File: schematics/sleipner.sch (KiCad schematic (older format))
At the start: 129 parts, among them J1 Conn_01x04_Male, J10 AudioJack3, J11 AudioJack3, J12 AudioJack3, J13 AudioJack3, J2 Barrel_Jack_Switch, J3 AudioJack3, J4 AudioJack3, J5 AudioJack3, J6 AudioJack3, J7 AudioJack3, J8 AudioJack3, J9 AudioJack3, Q1 BC337, Q2 BC337, Q3 BC337, Q4 BC337, Q5 BC337, Q6 BC337, Q7 BC337, Q8 BC337, Q9 BC337, SW1 SW_DIP_x02, SW10 SW_DIP_x02, SW11 Rotary_Encoder, SW12 SW_DIP_x02, SW13 SW_DIP_x02, SW14 SW_DIP_x02, SW15 SW_DIP_x02, SW16 SW_DIP_x02, SW17 SW_DIP_x02, SW18 SW_DIP_x02, SW19 SW_DIP_x02, SW2 SW_DIP_x02, SW3 SW_DIP_x02, SW4 SW_DIP_x02, SW5 SW_DIP_x02, SW6 SW_DIP_x02, SW7 SW_DIP_x02, SW8 SW_DIP_x02, SW9 SW_DIP_x02, U1 L7805, U2 ATmega32-16PU, U3 L7812, U4 74LS259, U5 MCP4922-EP, U6 TLC274, Y1 16 MHz

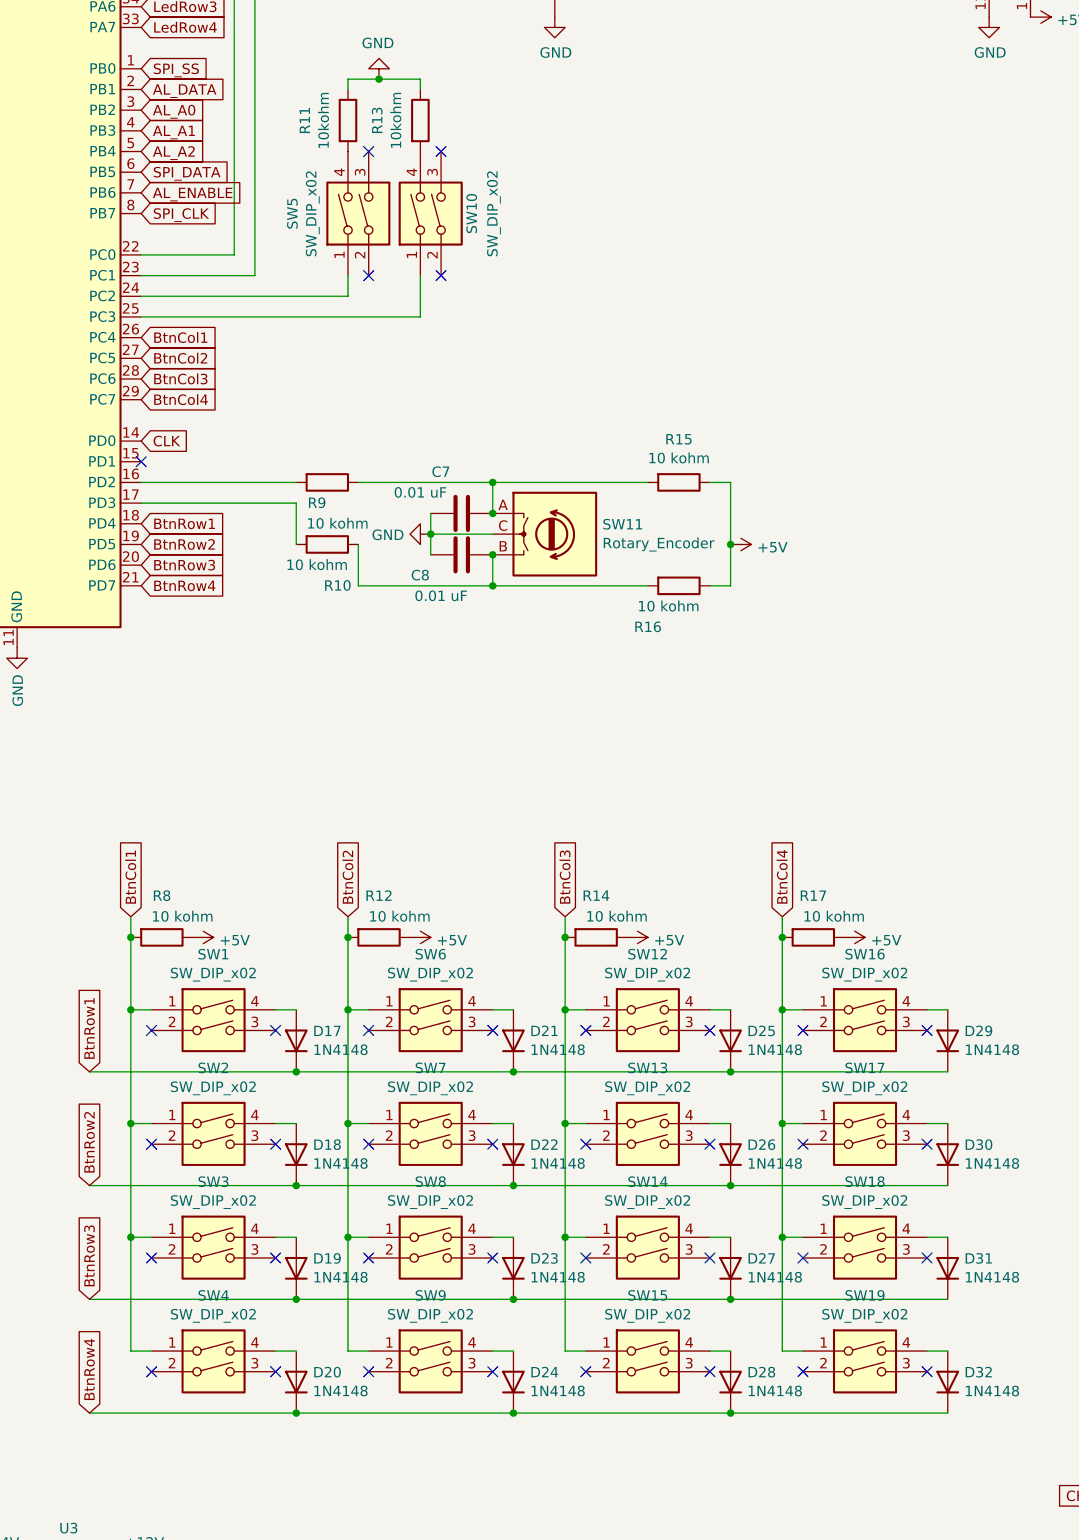
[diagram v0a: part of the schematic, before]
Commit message: Update schematics and add PCB layout
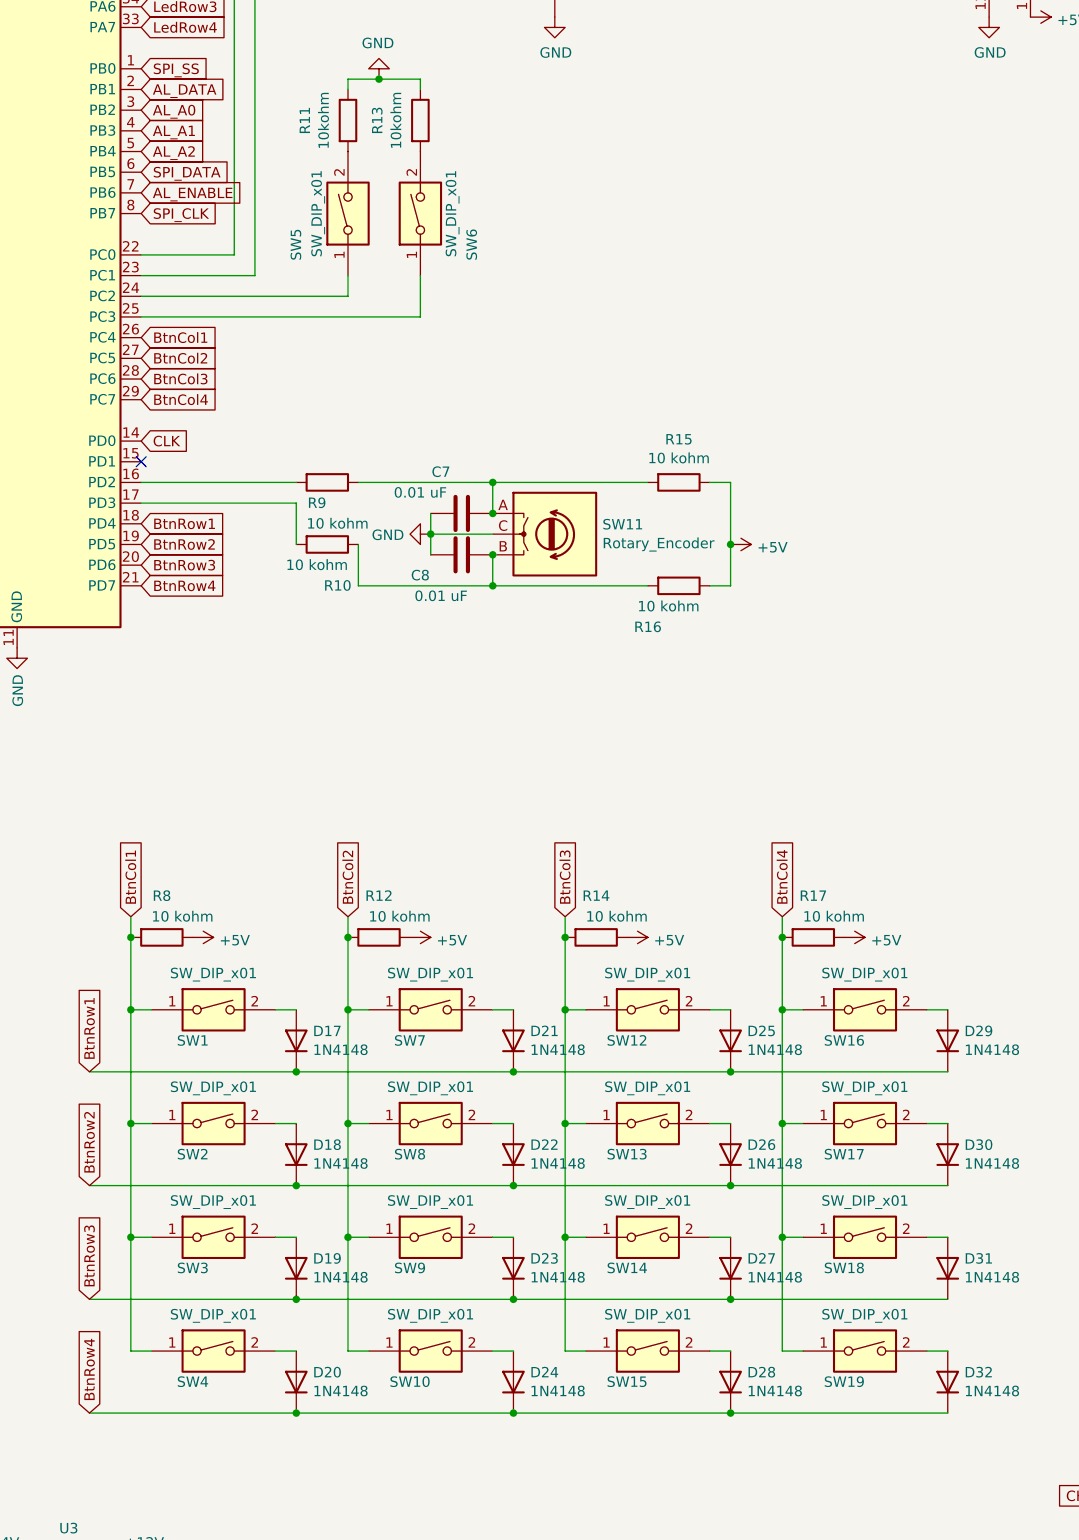
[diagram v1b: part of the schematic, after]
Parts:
- removed SW1, SW10, SW12, SW13, SW14, SW15, SW16, SW17, SW18, SW19, SW2, SW3, SW4, SW5, SW6, SW7, SW8, SW9: SW_DIP_x02, Button_Switch_THT:SW_PUSH-12mm, symbol Switch:SW_DIP_x02
- added SW1, SW10, SW12, SW13, SW14, SW15, SW16, SW17, SW18, SW19, SW2, SW3, SW4, SW5, SW6, SW7, SW8, SW9: SW_DIP_x01, Button_Switch_THT:SW_PUSH-12mm, symbol Switch:SW_DIP_x01
- J10, J11, J12, J13, J3, J4, J5, J6, J7, J8, J9: footprint (none) -> 3.5mmJack:3.55mmJack
- U4: footprint (none) -> Package_DIP:DIP-16_W7.62mm
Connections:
- net BtnCol1: now also SW1.1, SW2.1, SW3.1, SW4.1
- net BtnCol2: now also SW10.1, SW7.1, SW8.1, SW9.1
- net BtnCol3: now also SW12.1, SW13.1, SW14.1, SW15.1
- net BtnCol4: now also SW16.1, SW17.1, SW18.1, SW19.1
- net at U2.24 (PC2): now also SW5.1
- net at U2.25 (PC3): now also SW6.1
- net at D21.2 (A): now also SW7.2
- net at D17.2 (A): now also SW1.2
- net at D25.2 (A): now also SW12.2
- net at D29.2 (A): now also SW16.2
- net at D19.2 (A): now also SW3.2
- net at D23.2 (A): now also SW9.2
- net at D27.2 (A): now also SW14.2
- net at D31.2 (A): now also SW18.2
- net at D18.2 (A): now also SW2.2
- net at D22.2 (A): now also SW8.2
- net at D26.2 (A): now also SW13.2
- net at D30.2 (A): now also SW17.2
- net at D20.2 (A): now also SW4.2
- net at D24.2 (A): now also SW10.2
- net at D28.2 (A): now also SW15.2
- net at D32.2 (A): now also SW19.2
- net at R11.2: now also SW5.2
- net at R13.2: now also SW6.2
- no-connect marks 51 -> 15

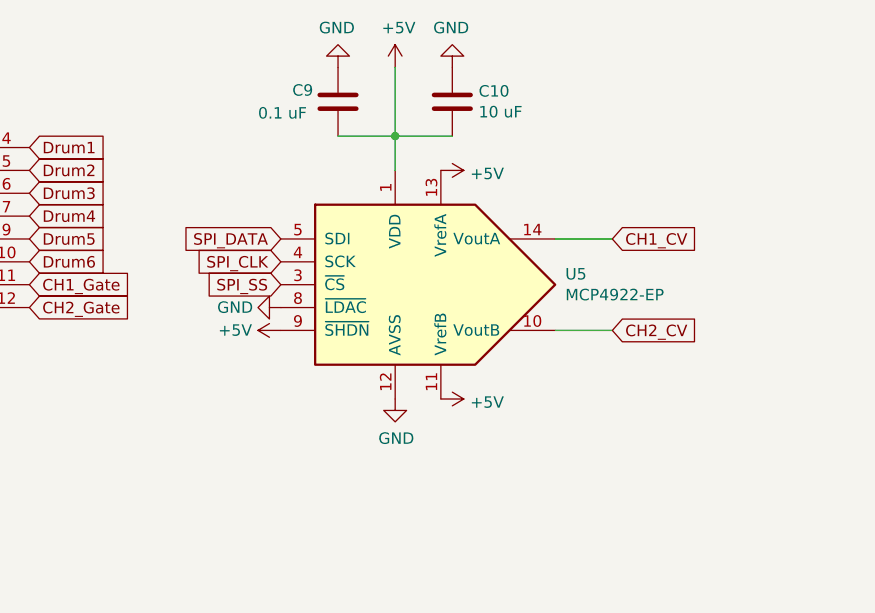
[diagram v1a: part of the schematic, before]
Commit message: Redo the PCB
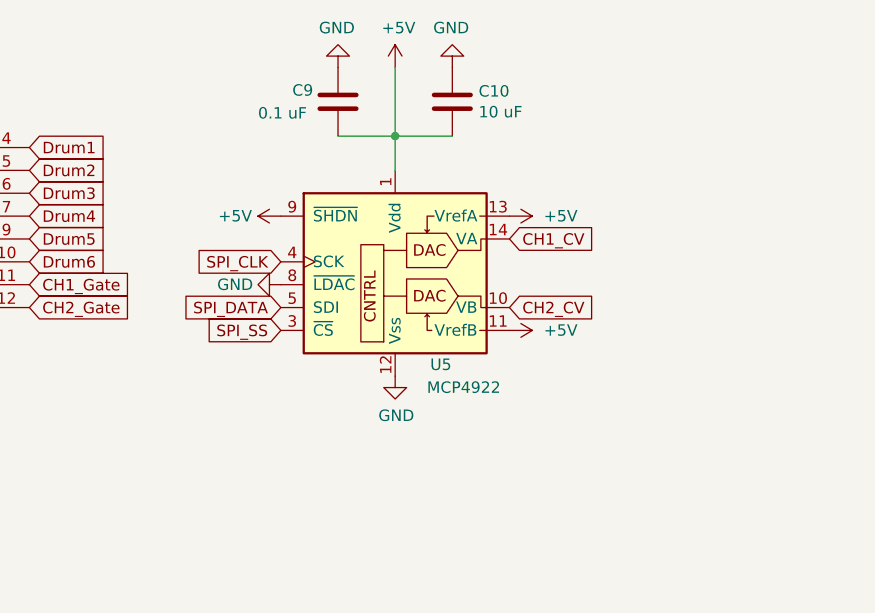
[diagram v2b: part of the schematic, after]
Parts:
- removed U5: MCP4922-EP, mcp4922:DIP254P762X533-14, symbol Analog_DAC:MCP4922-EP
- added U5: MCP4922, Package_DIP:DIP-14_W7.62mm, symbol Analog_DAC:MCP4922
- U6: footprint tlc274:DIP794W45P254L1969H508Q14 -> Package_DIP:DIP-14_W7.62mm
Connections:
- net +5V: now also U5.1 (Vdd), U5.11 (VrefB), U5.13 (VrefA), U5.9 (~SHDN)
- net CH1_CV: now also U5.14 (VA)
- net CH2_CV: now also U5.10 (VB)
- net GND: now also U5.12 (Vss), U5.8 (~LDAC)
- net SPI_CLK: now also U5.4 (SCK)
- net SPI_DATA: now also U5.5 (SDI)
- net SPI_SS: now also U5.3 (~CS)
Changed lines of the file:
@@
-$EndComp
-$Comp
-L Analog_DAC:MCP4922-EP U5
-U 1 1 60919F79
-P 7800 2350
-F 0 "U5" H 8444 2396 50  0000 L CNN
-F 1 "MCP4922-EP" H 8444 2305 50  0000 L CNN
-F 2 "mcp4922:DIP254P762X533-14" H 7800 2350 50  0001 C CIN
-F 3 "http://ww1.microchip.com/downloads/en/devicedoc/21897a.pdf" H 7800 2350 50  0001 C CNN
-	1    7800 2350
-	1    0    0    -1
 $EndComp
 $Comp
@@
 F 0 "U6" H 8750 10400 50  0000 C CNN
 F 1 "TLC274" H 8800 10300 50  0000 C CNN
-F 2 "tlc274:DIP794W45P254L1969H508Q14" H 8650 10200 50  0001 C CNN
+F 2 "Package_DIP:DIP-14_W7.62mm" H 8650 10200 50  0001 C CNN
 F 3 "http://www.ti.com/lit/ds/symlink/tlc274.pdf" H 8750 10300 50  0001 C CNN
 	1    8700 10100
@@
 F 0 "U6" H 8658 10146 50  0000 L CNN
 F 1 "TLC274" H 8658 10055 50  0000 L CNN
-F 2 "tlc274:DIP794W45P254L1969H508Q14" H 8650 10200 50  0001 C CNN
+F 2 "Package_DIP:DIP-14_W7.62mm" H 8650 10200 50  0001 C CNN
 F 3 "http://www.ti.com/lit/ds/symlink/tlc274.pdf" H 8750 10300 50  0001 C CNN
 	5    8700 10100
@@
 F 0 "U6" H 10500 10400 50  0000 C CNN
 F 1 "TLC274" H 10550 10300 50  0000 C CNN
-F 2 "tlc274:DIP794W45P254L1969H508Q14" H 10400 10200 50  0001 C CNN
+F 2 "Package_DIP:DIP-14_W7.62mm" H 10400 10200 50  0001 C CNN
 F 3 "http://www.ti.com/lit/ds/symlink/tlc274.pdf" H 10500 10300 50  0001 C CNN
 	2    10450 10100
@@
 L power:GND #PWR030
 U 1 1 6149602B
-P 7700 2850
-F 0 "#PWR030" H 7700 2600 50  0001 C CNN
-F 1 "GND" H 7705 2677 50  0000 C CNN
-F 2 "" H 7700 2850 50  0001 C CNN
-F 3 "" H 7700 2850 50  0001 C CNN
-	1    7700 2850
+P 7700 2750
+F 0 "#PWR030" H 7700 2500 50  0001 C CNN
+F 1 "GND" H 7705 2577 50  0000 C CNN
+F 2 "" H 7700 2750 50  0001 C CNN
+F 3 "" H 7700 2750 50  0001 C CNN
+	1    7700 2750
 	1    0    0    -1
 $EndComp
@@
 $EndComp
 $Comp
-L power:GND #PWR033
+L power:GND #PWR031
 U 1 1 6157DF10
 P 7950 1400
-F 0 "#PWR033" H 7950 1150 50  0001 C CNN
+F 0 "#PWR031" H 7950 1150 50  0001 C CNN
 F 1 "GND" H 7955 1227 50  0000 C CNN
 F 2 "" H 7950 1400 50  0001 C CNN
@@
 	1    0    0    -1
 $EndComp
-Text GLabel 8650 2150 2    50   Input ~ 0
+Text GLabel 8200 2150 2    50   Input ~ 0
 CH1_CV
-Text GLabel 8650 2550 2    50   Input ~ 0
+Text GLabel 8200 2450 2    50   Input ~ 0
 CH2_CV
 Text GLabel 14400 4600 1    50   Input ~ 0
@@
 Text GLabel 8400 10000 0    50   Input ~ 0
 CH1_CV
-Wire Wire Line
-	8400 2550 8650 2550
-Wire Wire Line
-	8400 2150 8650 2150
-$Comp
-L power:+5V #PWR031
+$Comp
+L power:+5V #PWR032
 U 1 1 63C2EF82
-P 7900 1850
-F 0 "#PWR031" H 7900 1700 50  0001 C CNN
-F 1 "+5V" V 7915 1978 50  0000 L CNN
-F 2 "" H 7900 1850 50  0001 C CNN
-F 3 "" H 7900 1850 50  0001 C CNN
-	1    7900 1850
-	0    1    1    0
-$EndComp
-$Comp
-L power:+5V #PWR032
+P 8200 2050
+F 0 "#PWR032" H 8200 1900 50  0001 C CNN
+F 1 "+5V" V 8200 2200 50  0000 L CNN
+F 2 "" H 8200 2050 50  0001 C CNN
+F 3 "" H 8200 2050 50  0001 C CNN
+	1    8200 2050
+	0    1    1    0
+$EndComp
+$Comp
+L power:+5V #PWR033
 U 1 1 63C4DC09
-P 7900 2850
-F 0 "#PWR032" H 7900 2700 50  0001 C CNN
-F 1 "+5V" V 7915 2978 50  0000 L CNN
-F 2 "" H 7900 2850 50  0001 C CNN
-F 3 "" H 7900 2850 50  0001 C CNN
-	1    7900 2850
+P 8200 2550
+F 0 "#PWR033" H 8200 2400 50  0001 C CNN
+F 1 "+5V" V 8200 2700 50  0000 L CNN
+F 2 "" H 8200 2550 50  0001 C CNN
+F 3 "" H 8200 2550 50  0001 C CNN
+	1    8200 2550
 	0    1    1    0
 $EndComp
@@
 	7700 1400 7700 1700
 $Comp
-L power:GND #PWR026
+L power:GND #PWR027
 U 1 1 60B62D9D
-P 7200 2450
-F 0 "#PWR026" H 7200 2200 50  0001 C CNN
-F 1 "GND" V 7200 2250 50  0000 C CNN
-F 2 "" H 7200 2450 50  0001 C CNN
-F 3 "" H 7200 2450 50  0001 C CNN
-	1    7200 2450
-	0    1    1    0
-$EndComp
-$Comp
-L power:+5V #PWR027
+P 7200 2350
+F 0 "#PWR027" H 7200 2100 50  0001 C CNN
+F 1 "GND" V 7200 2150 50  0000 C CNN
+F 2 "" H 7200 2350 50  0001 C CNN
+F 3 "" H 7200 2350 50  0001 C CNN
+	1    7200 2350
+	0    1    1    0
+$EndComp
+$Comp
+L power:+5V #PWR026
 U 1 1 60B64956
-P 7200 2550
-F 0 "#PWR027" H 7200 2400 50  0001 C CNN
-F 1 "+5V" V 7200 2750 50  0000 C CNN
-F 2 "" H 7200 2550 50  0001 C CNN
-F 3 "" H 7200 2550 50  0001 C CNN
-	1    7200 2550
+P 7200 2050
+F 0 "#PWR026" H 7200 1900 50  0001 C CNN
+F 1 "+5V" V 7200 2250 50  0000 C CNN
+F 2 "" H 7200 2050 50  0001 C CNN
+F 3 "" H 7200 2050 50  0001 C CNN
+	1    7200 2050
 	0    -1   -1   0
 $EndComp
-Text GLabel 7200 2150 0    50   Input ~ 0
+Text GLabel 7200 2450 0    50   Input ~ 0
 SPI_DATA
 Text GLabel 7200 2250 0    50   Input ~ 0
 SPI_CLK
-Text GLabel 7200 2350 0    50   Input ~ 0
+Text GLabel 7200 2550 0    50   Input ~ 0
 SPI_SS
 Text GLabel 3600 3800 2    50   Input ~ 0
@@
 	0    -1   -1   0
 $EndComp
+$Comp
+L Analog_DAC:MCP4922 U5
+U 1 1 60B2F9C3
+P 7700 2250
+F 0 "U5" H 7900 1800 50  0000 C CNN
+F 1 "MCP4922" H 8000 1700 50  0000 C CNN
+F 2 "Package_DIP:DIP-14_W7.62mm" H 8500 1950 50  0001 C CNN
+F 3 "http://ww1.microchip.com/downloads/en/DeviceDoc/22250A.pdf" H 8500 1950 50  0001 C CNN
+	1    7700 2250
+	1    0    0    -1
+$EndComp
 $EndSCHEMATC
